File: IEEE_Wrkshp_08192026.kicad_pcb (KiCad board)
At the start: 2 copper layers, 113 x 33.6 mm, 14 parts, among them J2 Screw_Terminal_01x02, J3 Screw_Terminal_01x02, Q1 2SD600, U2 TLV172IDCK

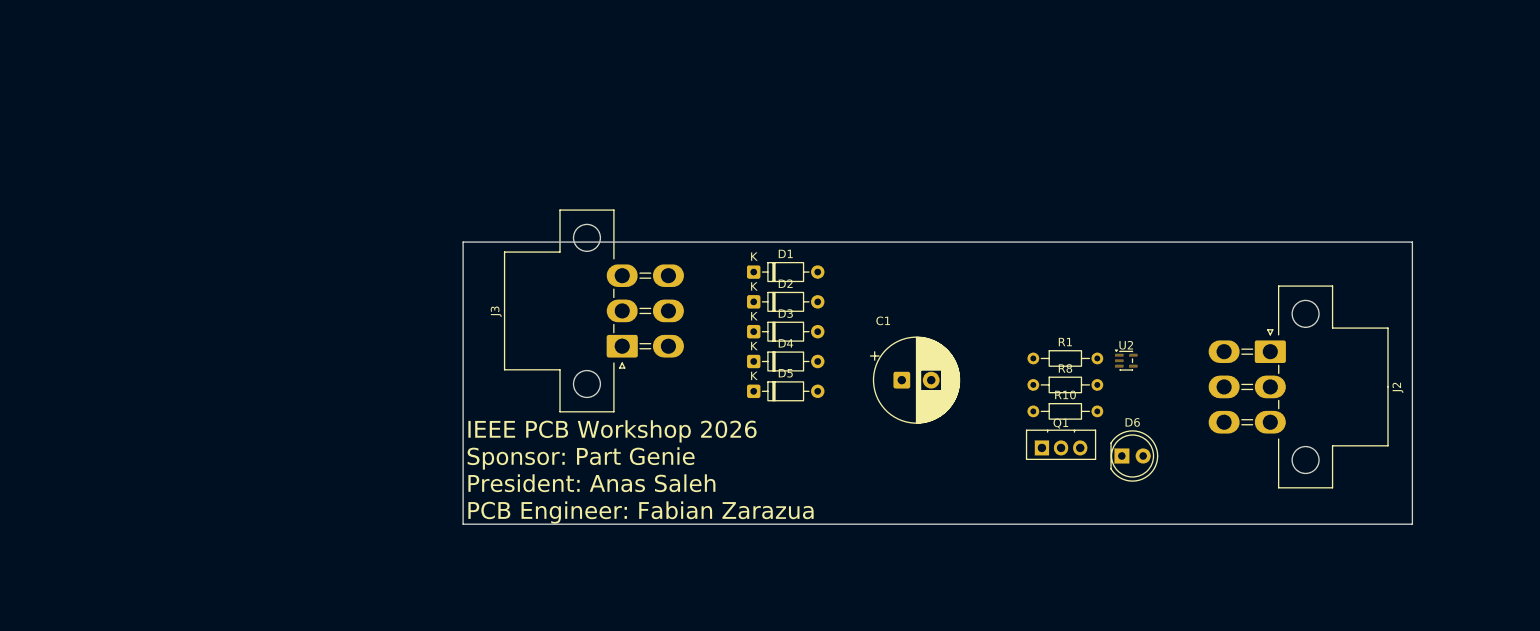
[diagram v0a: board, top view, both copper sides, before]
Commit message: 9/2 - Layout and Schematic
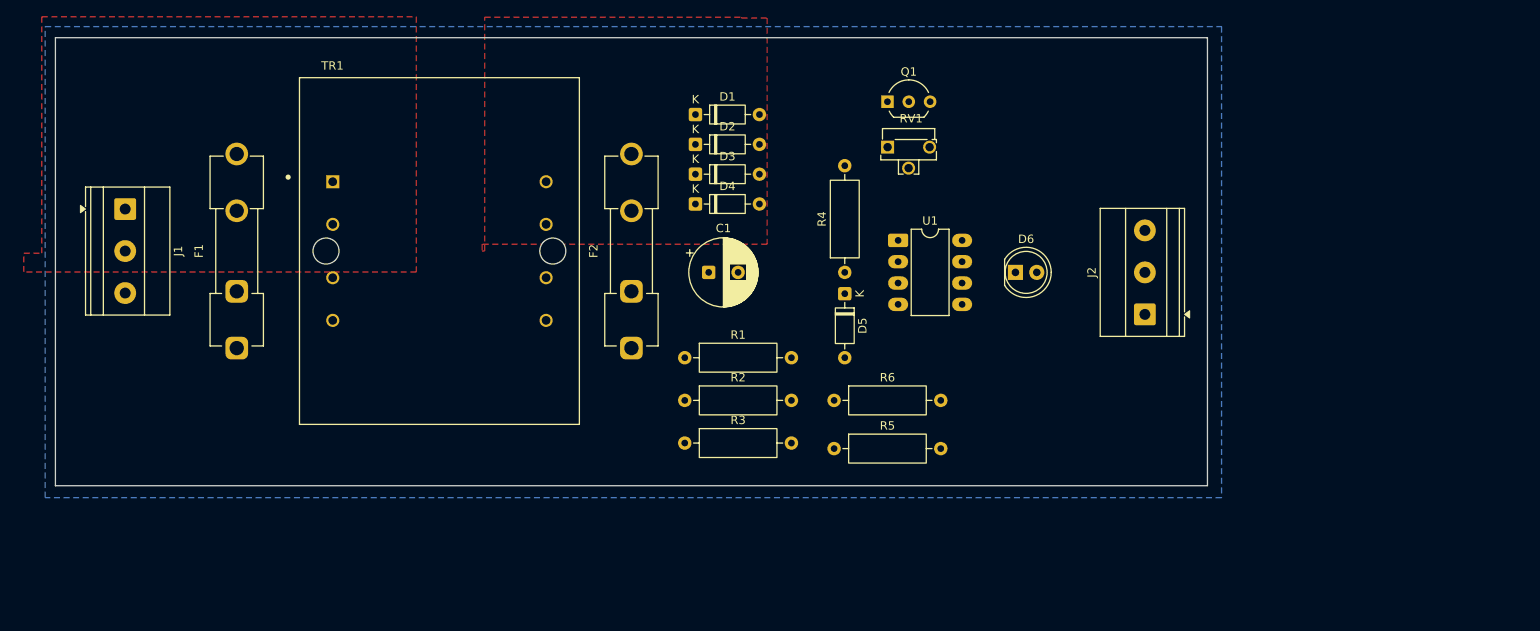
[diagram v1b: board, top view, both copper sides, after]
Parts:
- removed J3: Screw_Terminal_01x02, Connector_Molex:Molex_Mini-Fit_Jr_5569-06A1_2x03_P4.20mm_Horizontal
- removed R10, R8: R_US, Resistor_THT:R_Axial_DIN0204_L3.6mm_D1.6mm_P7.62mm_Horizontal
- removed U2: TLV172IDCK, Package_TO_SOT_SMD:SOT-353_SC-70-5
- added F1: 100mA, Fuse:Fuseholder_Clip-5x20mm_Keystone_3517_Inline_P23.11x6.76mm_D1.70mm_Horizontal, F.Cu at (67.3, 95.4)
- added F2: 1A, Fuse:Fuseholder_Clip-5x20mm_Keystone_3517_Inline_P23.11x6.76mm_D1.70mm_Horizontal, F.Cu at (114.3, 95.4)
- added J1: Screw_Terminal_01x03, TerminalBlock_Phoenix:TerminalBlock_Phoenix_MKDS-1,5-3_1x03_P5.00mm_Horizontal, F.Cu at (54.0, 78.8)
- added R2: 0, Resistor_THT:R_Axial_DIN0309_L9.0mm_D3.2mm_P12.70mm_Horizontal, F.Cu at (120.7, 101.6)
- added R3: 0, Resistor_THT:R_Axial_DIN0309_L9.0mm_D3.2mm_P12.70mm_Horizontal, F.Cu at (120.7, 106.7)
- added R4: 10k, Resistor_THT:R_Axial_DIN0309_L9.0mm_D3.2mm_P12.70mm_Horizontal, F.Cu at (139.7, 86.4)
- added R5: 680, Resistor_THT:R_Axial_DIN0309_L9.0mm_D3.2mm_P12.70mm_Horizontal, F.Cu at (138.4, 107.3)
- added R6: 220, Resistor_THT:R_Axial_DIN0309_L9.0mm_D3.2mm_P12.70mm_Horizontal, F.Cu at (138.4, 101.6)
- added RV1: 10k, Potentiometer_THT:Potentiometer_Runtron_RM-063_Horizontal, F.Cu at (144.8, 71.5)
- added TR1: VPP12-200, Transformer_THT:XFMR_VPP12-200, F.Cu at (91.4, 83.8)
- added U1: TLV172IDCK, Package_DIP:DIP-8_W7.62mm_LongPads, F.Cu at (146.1, 82.5)
- C1: footprint Capacitor_THT:CP_Radial_D10.0mm_P3.50mm -> Capacitor_THT:CP_Radial_D8.0mm_P3.50mm
- D5: value D_Zener -> 1V
- D6: value LED -> Red
- J2: value Screw_Terminal_01x02 -> Screw_Terminal_01x03; footprint Connector_Molex:Molex_Mini-Fit_Jr_5569-06A1_2x03_P4.20mm_Horizontal -> TerminalBlock_Phoenix:TerminalBlock_Phoenix_MKDS-1,5-3_1x03_P5.00mm_Horizontal
- Q1: footprint Package_TO_SOT_THT:TO-126-3_Vertical -> Package_TO_SOT_THT:TO-92_Inline_Wide
- R1: value R_US -> 0; footprint Resistor_THT:R_Axial_DIN0204_L3.6mm_D1.6mm_P7.62mm_Horizontal -> Resistor_THT:R_Axial_DIN0309_L9.0mm_D3.2mm_P12.70mm_Horizontal
- moved Q1 45.1 mm to (144.8, 66.0)
- moved R1 41.5 mm to (120.7, 96.5)
- moved C1 26.3 mm to (123.5, 86.4)
- moved D6 25.3 mm to (160.0, 86.4)
- moved D1 20.0 mm to (121.9, 67.6)
- moved D2 20.0 mm to (121.9, 71.1)
- moved D3 20.0 mm to (121.9, 74.7)
- moved D4 20.0 mm to (121.9, 78.2)
- moved D5 15.9 mm to (139.7, 88.9), turned to -90 degrees
- moved J2 15.6 mm to (175.4, 91.4), turned to 90 degrees
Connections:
- net Net-(D6-A) renamed /Vout
- C1 pad 2: /AC_Rectified_V- -> GND2
- D1 pad 2: /AC_Rectified_V- -> GND2
- D2 pad 1: /T2 -> GND2
- D2 pad 2: /AC_Rectified_V- -> GND2
- D4 pad 2: /T2 -> GND2
- D5 pad 1: Net-(D5-K) -> /VRef
- D5 pad 2: /AC_Rectified_V- -> GND2
- J2 pad 2: /AC_Rectified_V- -> GND2
- J2 pad 3: (no net) -> GND1
- R1 pad 1: /AC_Rectified_V+ -> /C1-
- R1 pad 2: Net-(D5-K) -> GND2
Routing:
- added copper zone on F.Cu, net /AC_Rectified_V+
- added copper zone on F.Cu, net /T1
- added copper zone on B.Cu, net GND2
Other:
- board size 113 x 33.6 mm -> 137.2 x 53.3 mm
- board text added: "IEEE Workshop 2026 PCB Design Series President: Anas Saleh PCB Engineer: Fabian Zarazua"
- board text removed: "IEEE PCB Workshop 2026 Sponsor: Part Genie President: Anas Saleh PCB Engineer: Fabian Zarazua"

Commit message: Almost Done
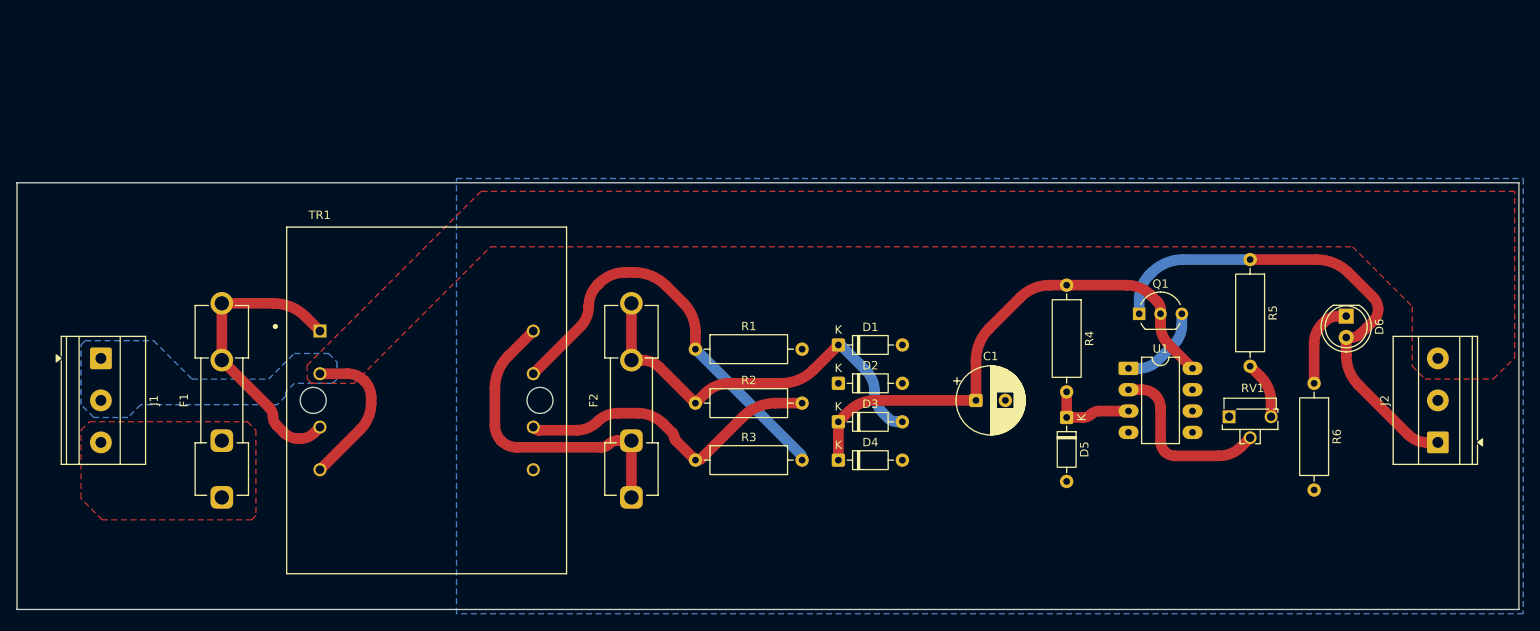
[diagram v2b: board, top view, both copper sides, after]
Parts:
- J1: value Screw_Terminal_01x03 -> TB002-500-02BE
- Q1: value 2SD600 -> BC63916-D27Z
- U1: value TLV172IDCK -> LM358P
- moved R6 57.2 mm to (195.6, 99.6), turned to -90 degrees
- moved R5 54.4 mm to (188.0, 84.8), turned to -90 degrees
- moved RV1 51.8 mm to (185.5, 103.5)
- moved D6 39.7 mm to (199.4, 91.6), turned to -90 degrees
- moved Q1 39.2 mm to (174.8, 91.3)
- moved J2 38.1 mm to (210.3, 106.6)
- moved C1 35.3 mm to (155.3, 101.6)
- moved D4 34.9 mm to (138.9, 108.7)
- moved D3 34.0 mm to (138.9, 104.2)
- moved D2 33.1 mm to (138.9, 99.6)
- moved D1 32.3 mm to (138.9, 95.0)
- moved U1 31.4 mm to (173.5, 97.8)
- moved D5 30.2 mm to (166.1, 103.6)
- moved R4 26.5 mm to (166.1, 87.9), turned to -90 degrees
- moved J1 18.0 mm to (51.1, 96.6)
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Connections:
- net /AC_Pin1 renamed /+
- net /C1+ renamed /S1+
- net /C1- renamed /S1-
- net /C2+ renamed /S2+
- net /T1 renamed Net-(D1-K)
- C1 pad 2: GND2 -> GND1
- D1 pad 2: GND2 -> GND1
- D2 pad 1: GND2 -> GND1
- D2 pad 2: GND2 -> GND1
- D4 pad 2: GND2 -> GND1
- D5 pad 2: GND2 -> GND1
- J1 pad 1: GND1 -> GNDPWR
- J1 pad 2: GND1 -> GNDPWR
- J2 pad 2: GND2 -> GND1
- J2 pad 3: GND1 -> GNDPWR
- R1 pad 2: GND2 -> GND1
- R6 pad 2: GND2 -> GND1
- RV1 pad 1: GND2 -> GND1
- TR1 pad 2: GND1 -> GNDPWR
- TR1 pad 4: GND1 -> GNDPWR
- TR1 pad 5: GND2 -> GND1
- U1 pad 1: /VRef -> Net-(Q1-B)
- U1 pad 2: GND2 -> /Vfdbck
- U1 pad 3: /Vfdbck -> /VRef
- U1 pad 4: Net-(Q1-B) -> GND1
- U1 pad 5: /AC_Rectified_V+ -> unconnected-(U1-Pad5)
- U1 pad 6: (no net) -> unconnected-(U1-Pad6)
- U1 pad 7: (no net) -> unconnected-(U1-Pad7)
- U1 pad 8: (no net) -> /AC_Rectified_V+
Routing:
- net /AC_Rectified_V+: track 0.00 -> 62.7 mm
- net /Vout: track 0.00 -> 58.9 mm
- net /S1-: track 0.00 -> 49.6 mm, vias 0 -> 1
- net Net-(D1-K): track 0.00 -> 48.0 mm
- net /S1+: track 0.00 -> 37.5 mm, vias 0 -> 1
- net /S2+: track 0.00 -> 37.5 mm
- net Net-(F1-Pad2): track 0.00 -> 36.0 mm
- net /Vfdbck: track 0.00 -> 21.4 mm
- net GNDPWR: track 0.00 -> 18.6 mm
- net /VRef: track 0.00 -> 10.6 mm
- net Net-(D6-K): track 0.00 -> 10.4 mm
- net Net-(Q1-B): track 0.00 -> 10.3 mm
- net Net-(R5-Pad2): track 0.00 -> 6.85 mm
- added copper zone on F.Cu, net /+
- added copper zone on B.Cu, net GND1
- added copper zone on B.Cu, net GNDPWR
- added copper zone on F.Cu, net GNDPWR
- removed copper zone on F.Cu, net /AC_Rectified_V+
- removed copper zone on B.Cu, net GND2
- removed copper zone on F.Cu, net Net-(D1-K)
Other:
- board size 137.2 x 53.3 mm -> 178.8 x 50.8 mm
- board text added: "IEEE Workshop 2026 PCB Design Series"
- board text added: "President: Anas Saleh PCB Engineer: Fabian Zarazua Sponsor: PartGenie"
- board text removed: "IEEE Workshop 2026 PCB Design Series President: Anas Saleh PCB Engineer: Fabian Zarazua"
